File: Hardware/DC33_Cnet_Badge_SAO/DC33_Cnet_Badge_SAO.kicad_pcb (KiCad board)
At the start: 2 copper layers, 59.5 x 70.5 mm, 4 parts, among them J1 Conn_02x03_Top_Bottom

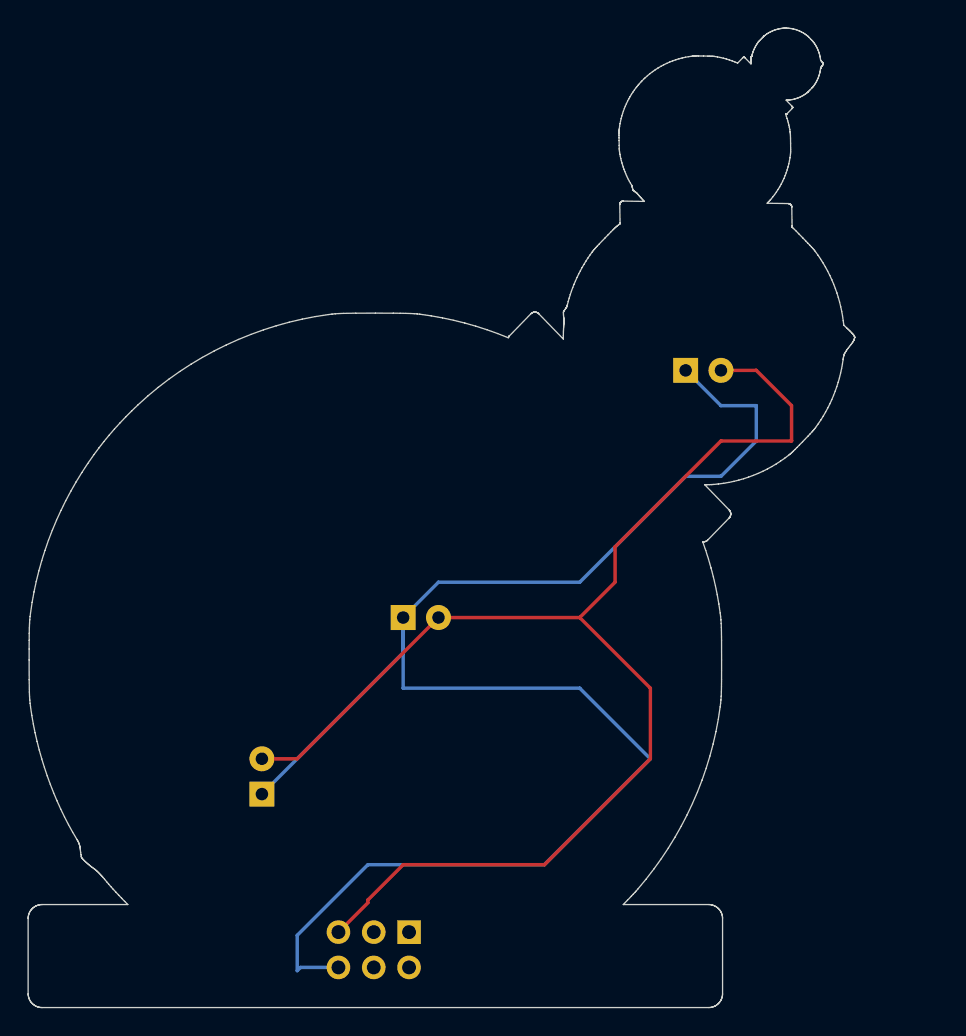
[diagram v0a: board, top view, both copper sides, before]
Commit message: SAO Updates
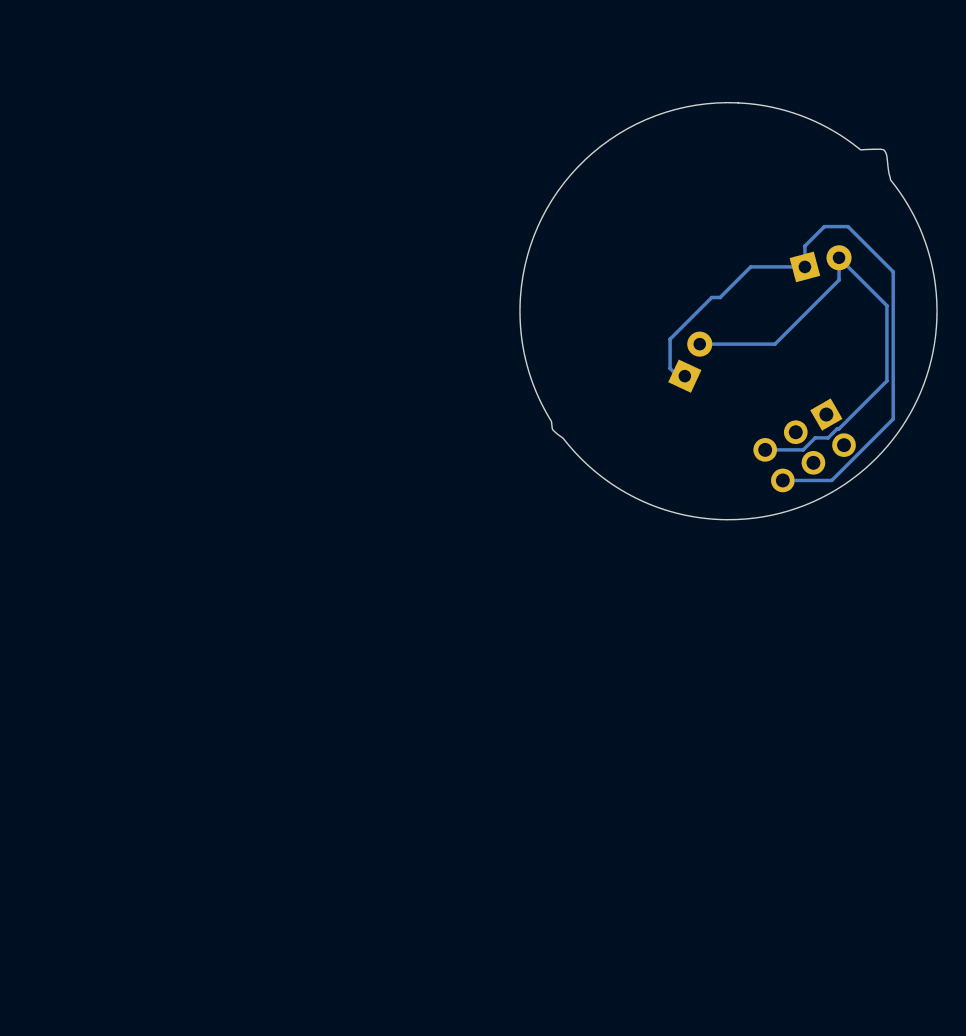
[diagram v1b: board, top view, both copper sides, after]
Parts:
- removed D3: LED, LED_THT:LED_D3.0mm
- added G***: LOGO, CactusCon_2025_CNet_SAO:Cnet_Logo_30x30, F.Cu at (150.0, 100.0)
- J1: footprint DC31_Cnet_Badge_SAO:PinSocket_2x03_P2.54mm_Vertical_Tab -> CactusCon_2025_CNet_SAO:PinSocket_2x03_P2.54mm_Vertical_Tab
- moved D1 54.4 mm to (155.9, 96.7), turned to 15 degrees
- moved J1 47.8 mm to (157.4, 107.3), turned to 120 degrees
- moved D2 26.7 mm to (147.3, 104.6), turned to 65 degrees
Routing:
- net GND: track 117.5 -> 45.4 mm
- net +3.3V: track 97.7 -> 34.6 mm
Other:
- board size 59.5 x 70.5 mm -> 30 x 30 mm
